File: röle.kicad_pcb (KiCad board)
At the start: 2 copper layers, 68.4 x 27.9 mm, 9 parts, among them J1 Conn_01x03_Pin, J2 Conn_01x03_Pin, K1 JQC-3F-1C-24VDC, U1 PC817

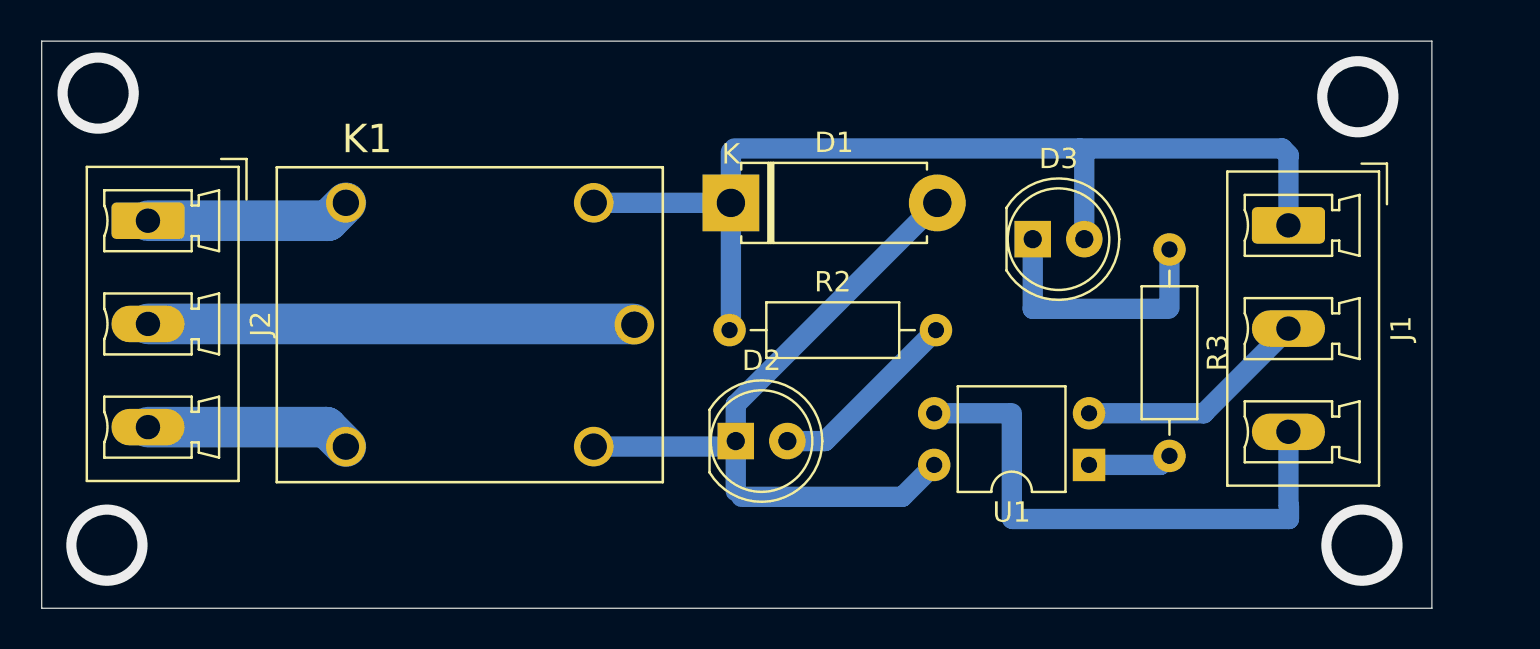
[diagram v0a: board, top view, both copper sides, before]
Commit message: Add files via upload
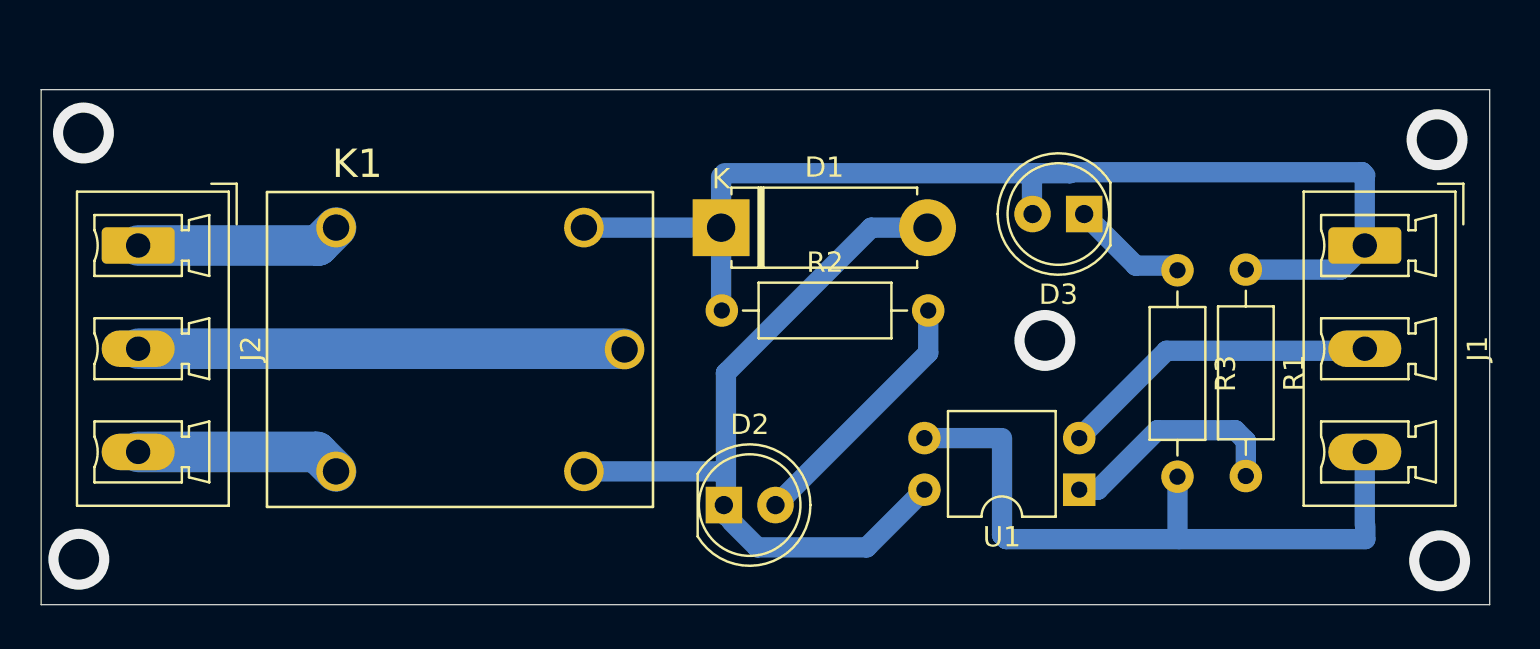
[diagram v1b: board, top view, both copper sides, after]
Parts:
- added R3: R, Resistor_THT:R_Axial_DIN0207_L6.3mm_D2.5mm_P10.16mm_Horizontal, F.Cu at (55.9, -16.4)
- moved J1 3.89 mm to (65.1, -17.6)
- moved R1 3.89 mm to (59.3, -16.4)
- moved D2 3.20 mm to (33.6, -4.85)
- moved D3 2.82 mm to (51.3, -19.2), turned to 180 degrees
- moved K1 1.31 mm to (20.6, -12.5)
- moved J2 1.31 mm to (4.75, -17.6)
- moved D1 1.31 mm to (33.4, -18.5)
- moved U1 1.31 mm to (51.1, -5.61)
- moved R2 1.04 mm to (33.5, -14.4)
- renumbered R3 to R1
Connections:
- R1 pad 1: Net-(D3-K) -> 12v
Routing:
- net GND: track 28.0 -> 35.4 mm
- net Net-(D3-K): track 13.1 -> 5.74 mm
- net Net-(R1-Pad2): track 4.14 -> 11.4 mm
- net 12v: track 51.3 -> 57.5 mm
- net in: track 11.8 -> 16.1 mm
- net Net-(D2-A): track 9.58 -> 12.7 mm
- net Net-(D1-A): track 35.9 -> 38.6 mm
- net (no net): vias 4 -> 5
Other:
- board size 68.4 x 27.9 mm -> 71.3 x 25.3 mm
